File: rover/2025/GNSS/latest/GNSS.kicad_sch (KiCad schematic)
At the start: 30 parts, among them J1 Eth-Horiz, J2 Eth-Horiz, J4 JST6_Pin, J5 USB_C_USB4145-GCT, SW1 TS09-63-25-WT-160-SMT-TR, SW2 TS09-63-25-WT-160-SMT-TR, U1 SN65HVD232, U2 ESP32-S3-WROVER, U3 LDO-LM7805MPX/NOPB, U4 LDO-TLV74033PDBVR, U5 TVS

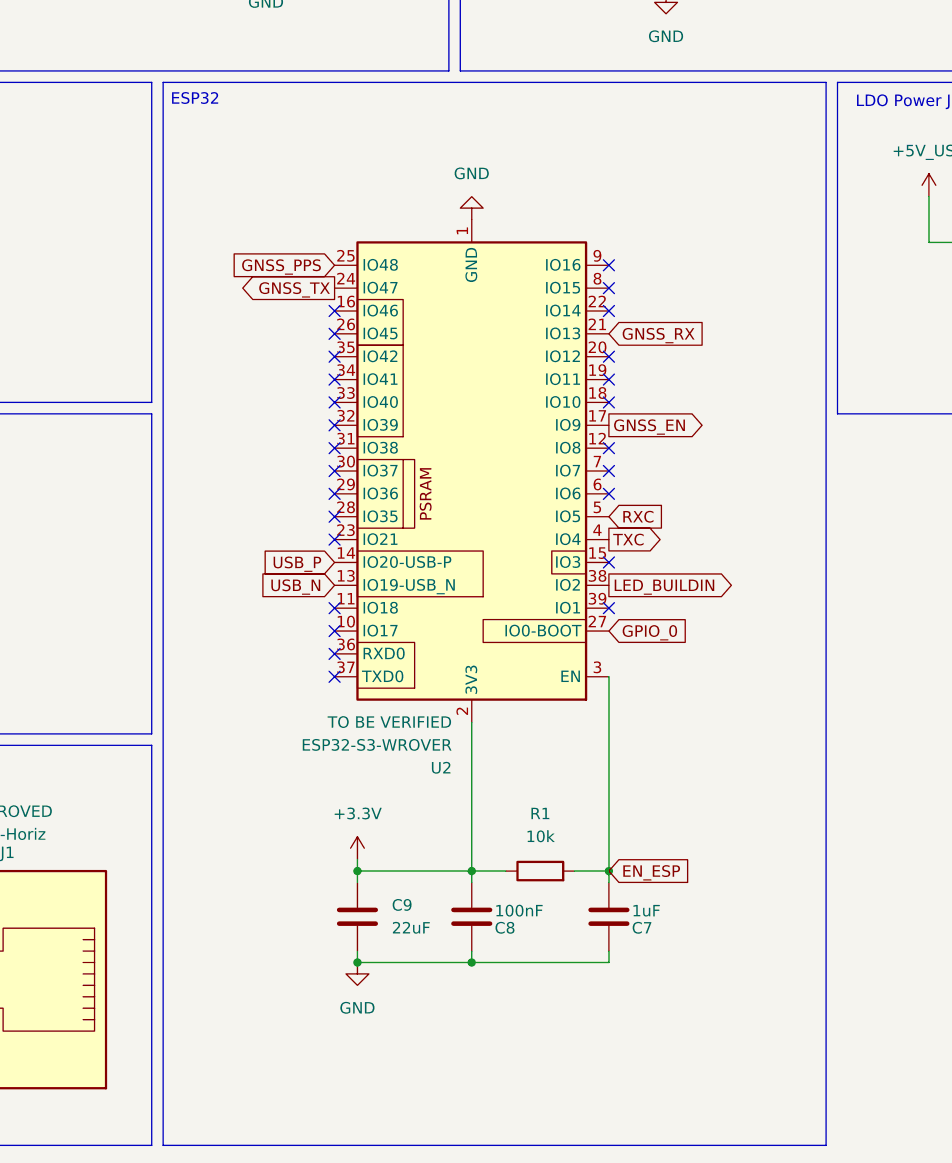
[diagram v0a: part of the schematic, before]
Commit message: GNSS Revision (Pas finit)
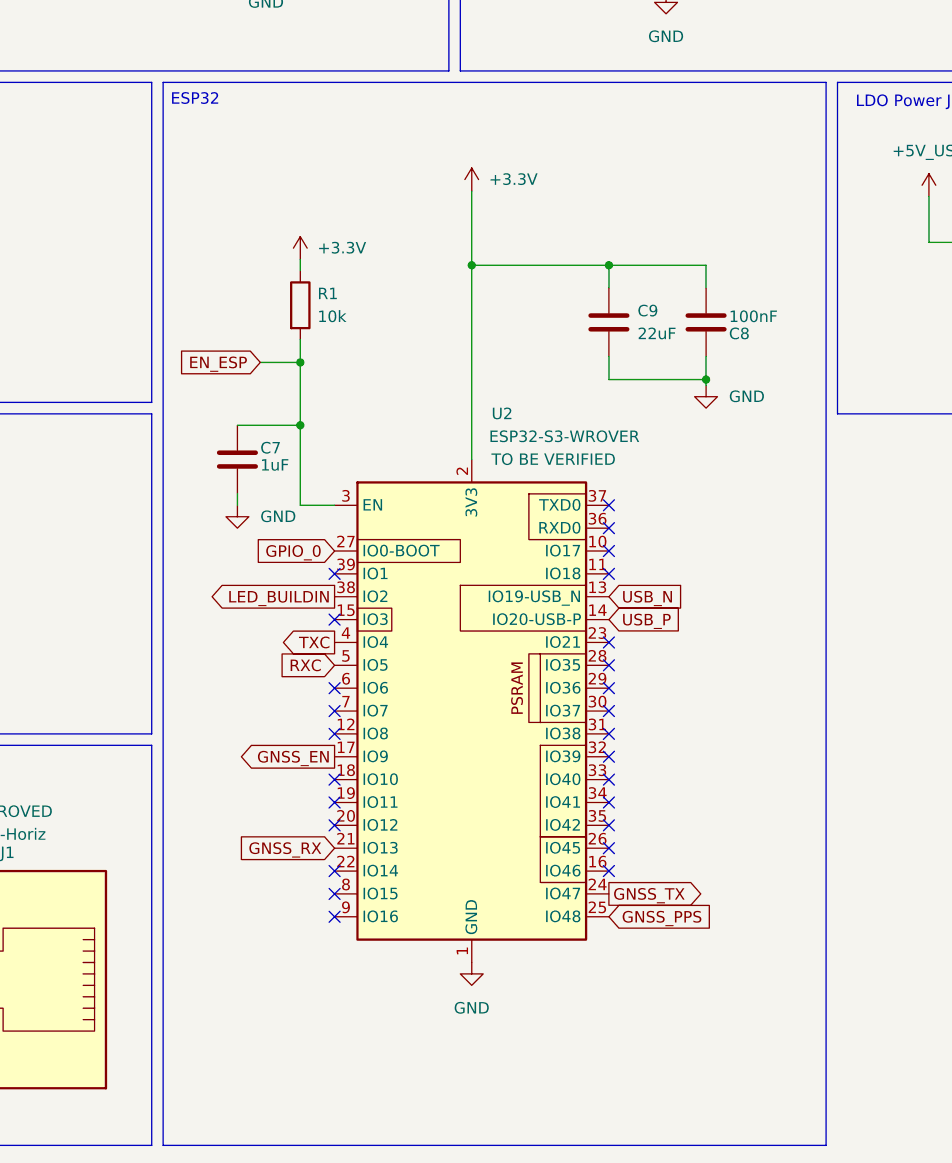
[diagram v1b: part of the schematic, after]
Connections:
- net EN_ESP: now also C7.1; no longer C7.2
- net GND: now also C7.2; no longer C7.1
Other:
- moved on the sheet: C7, C8, C9, R1, U2
